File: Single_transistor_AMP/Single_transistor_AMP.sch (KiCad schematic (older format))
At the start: 11 parts, among them J1 Signals ieeja, J2 Signals izeja, J3 12V, Q1 BC548

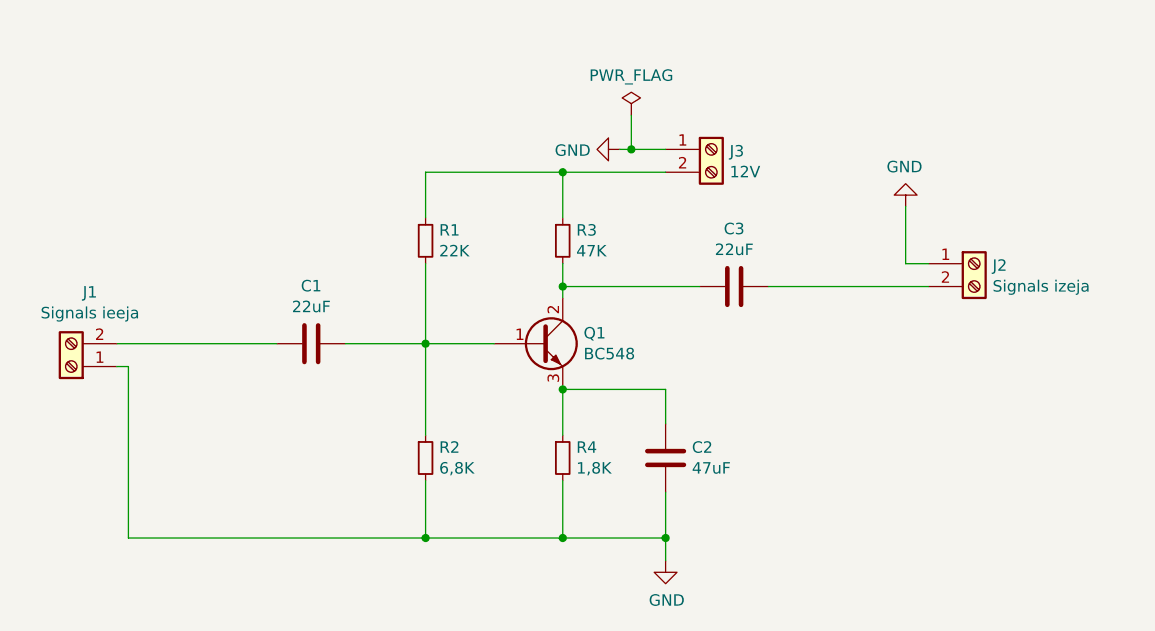
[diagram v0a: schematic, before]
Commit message: 3MD
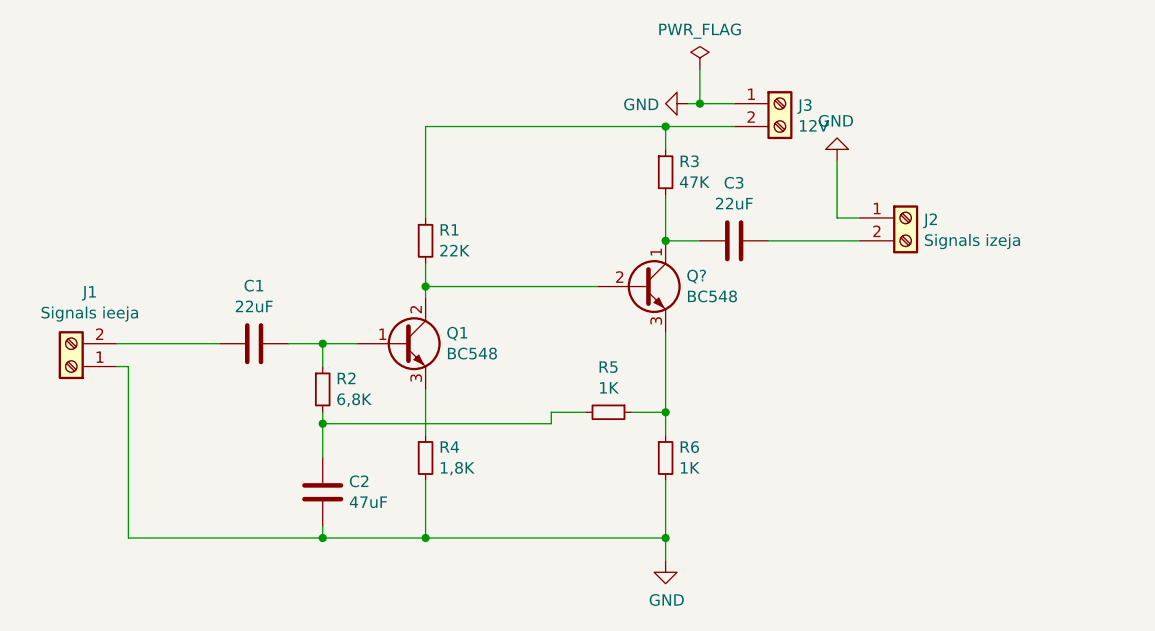
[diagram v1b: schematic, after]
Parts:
- added Q?: BC548, Package_TO_SOT_THT:TO-92_Inline, symbol Transistor_BJT:BC548
- added R5, R6: 1K, Resistor_SMD:R_0402_1005Metric, symbol Device:R_Small
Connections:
- net GND: now also R6.2; no longer R2.2
- net at C1.1, Q1.1 (B), R2.1: no longer R1.2
- net at C3.2, R3.2: now also Q?.1 (C); no longer Q1.2 (C)
- net at Q1.3 (E), R4.1: no longer C2.1
- new net: Q1.2 (C), Q?.2 (B), R1.2
- new net: C2.1, R2.2, R5.2
- new net: Q?.3 (E), R5.1, R6.1
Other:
- moved on the sheet: C1, C2, C3, J2, J3, Q1, R2, R3, R4
